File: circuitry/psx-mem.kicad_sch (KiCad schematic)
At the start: 27 parts, among them J1 Conn_01x08, J2 Conn_01x06, U1 PFS154-S16, U2 ZD25WQ16C

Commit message: Generated interactive bill of materials.
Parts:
- TP1, TP10, TP11, TP12, TP2, TP3, TP4, TP5, TP6, TP7, TP8, TP9: now left out of the parts list
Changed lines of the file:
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@@
 		(unit 1)
 		(exclude_from_sim no)
-		(in_bom yes)
+		(in_bom no)
 		(on_board yes)
 		(dnp no)
@@
 		(unit 1)
 		(exclude_from_sim no)
-		(in_bom yes)
+		(in_bom no)
 		(on_board yes)
 		(dnp no)
@@
 		(unit 1)
 		(exclude_from_sim no)
-		(in_bom yes)
+		(in_bom no)
 		(on_board yes)
 		(dnp no)
@@
 		(unit 1)
 		(exclude_from_sim no)
-		(in_bom yes)
+		(in_bom no)
 		(on_board yes)
 		(dnp no)
@@
 		(unit 1)
 		(exclude_from_sim no)
-		(in_bom yes)
+		(in_bom no)
 		(on_board yes)
 		(dnp no)
@@
 		(unit 1)
 		(exclude_from_sim no)
-		(in_bom yes)
+		(in_bom no)
 		(on_board yes)
 		(dnp no)
@@
 		(unit 1)
 		(exclude_from_sim no)
-		(in_bom yes)
+		(in_bom no)
 		(on_board yes)
 		(dnp no)
@@
 		(unit 1)
 		(exclude_from_sim no)
-		(in_bom yes)
+		(in_bom no)
 		(on_board yes)
 		(dnp no)
@@
 		(unit 1)
 		(exclude_from_sim no)
-		(in_bom yes)
+		(in_bom no)
 		(on_board yes)
 		(dnp no)
@@
 		(unit 1)
 		(exclude_from_sim no)
-		(in_bom yes)
+		(in_bom no)
 		(on_board yes)
 		(dnp no)
@@
 		(unit 1)
 		(exclude_from_sim no)
-		(in_bom yes)
+		(in_bom no)
 		(on_board yes)
 		(dnp no)
@@
 		(unit 1)
 		(exclude_from_sim no)
-		(in_bom yes)
-		(on_board yes)
-		(dnp no)
+		(in_bom no)
+		(on_board yes)
+		(dnp no)

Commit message: Updated to use libraries in submodules.
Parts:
- TP1, TP10, TP11, TP12, TP2, TP3, TP4, TP5, TP6, TP7, TP8, TP9: symbol PSX-MEM:TestPoint -> PSX_Memory:TestPoint; now in the parts list
- U1: symbol PSX-MEM:PFS154-S16 -> PSX_Memory:PFS154-S16
- U2: symbol PSX-MEM:ZD25WQ16V -> PSX_Memory:ZD25WQ16V
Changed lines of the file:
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@@
 	)
 	(symbol
-		(lib_id "PSX-MEM:TestPoint")
+		(lib_id "PSX_Memory:TestPoint")
 		(at 154.94 124.46 0)
 		(mirror x)
 		(unit 1)
 		(exclude_from_sim no)
-		(in_bom no)
+		(in_bom yes)
 		(on_board yes)
 		(dnp no)
@@
 	)
 	(symbol
-		(lib_id "PSX-MEM:TestPoint")
+		(lib_id "PSX_Memory:TestPoint")
 		(at 71.12 81.28 0)
 		(unit 1)
 		(exclude_from_sim no)
-		(in_bom no)
+		(in_bom yes)
 		(on_board yes)
 		(dnp no)
@@
 	)
 	(symbol
-		(lib_id "PSX-MEM:TestPoint")
+		(lib_id "PSX_Memory:TestPoint")
 		(at 139.7 124.46 0)
 		(mirror x)
 		(unit 1)
 		(exclude_from_sim no)
-		(in_bom no)
+		(in_bom yes)
 		(on_board yes)
 		(dnp no)
@@
 	)
 	(symbol
-		(lib_id "PSX-MEM:TestPoint")
+		(lib_id "PSX_Memory:TestPoint")
 		(at 78.74 81.28 0)
 		(unit 1)
 		(exclude_from_sim no)
-		(in_bom no)
+		(in_bom yes)
 		(on_board yes)
 		(dnp no)
@@
 	)
 	(symbol
-		(lib_id "PSX-MEM:ZD25WQ16V")
+		(lib_id "PSX_Memory:ZD25WQ16V")
 		(at 121.92 114.3 0)
 		(unit 1)
@@
 	)
 	(symbol
-		(lib_id "PSX-MEM:TestPoint")
+		(lib_id "PSX_Memory:TestPoint")
 		(at 86.36 124.46 180)
 		(unit 1)
 		(exclude_from_sim no)
-		(in_bom no)
+		(in_bom yes)
 		(on_board yes)
 		(dnp no)
@@
 	)
 	(symbol
-		(lib_id "PSX-MEM:TestPoint")
+		(lib_id "PSX_Memory:TestPoint")
 		(at 147.32 124.46 0)
 		(mirror x)
 		(unit 1)
 		(exclude_from_sim no)
-		(in_bom no)
+		(in_bom yes)
 		(on_board yes)
 		(dnp no)
@@
 	)
 	(symbol
-		(lib_id "PSX-MEM:TestPoint")
+		(lib_id "PSX_Memory:TestPoint")
 		(at 63.5 124.46 0)
 		(mirror x)
 		(unit 1)
 		(exclude_from_sim no)
-		(in_bom no)
+		(in_bom yes)
 		(on_board yes)
 		(dnp no)
@@
 	)
 	(symbol
-		(lib_id "PSX-MEM:TestPoint")
+		(lib_id "PSX_Memory:TestPoint")
 		(at 71.12 124.46 0)
 		(mirror x)
 		(unit 1)
 		(exclude_from_sim no)
-		(in_bom no)
+		(in_bom yes)
 		(on_board yes)
 		(dnp no)
@@
 	)
 	(symbol
-		(lib_id "PSX-MEM:TestPoint")
+		(lib_id "PSX_Memory:TestPoint")
 		(at 162.56 124.46 0)
 		(mirror x)
 		(unit 1)
 		(exclude_from_sim no)
-		(in_bom no)
+		(in_bom yes)
 		(on_board yes)
 		(dnp no)
@@
 	)
 	(symbol
-		(lib_id "PSX-MEM:TestPoint")
+		(lib_id "PSX_Memory:TestPoint")
 		(at 93.98 124.46 180)
 		(unit 1)
 		(exclude_from_sim no)
-		(in_bom no)
+		(in_bom yes)
 		(on_board yes)
 		(dnp no)
@@
 	)
 	(symbol
-		(lib_id "PSX-MEM:TestPoint")
+		(lib_id "PSX_Memory:TestPoint")
 		(at 63.5 81.28 0)
 		(unit 1)
 		(exclude_from_sim no)
-		(in_bom no)
+		(in_bom yes)
 		(on_board yes)
 		(dnp no)
@@
 	)
 	(symbol
-		(lib_id "PSX-MEM:TestPoint")
+		(lib_id "PSX_Memory:TestPoint")
 		(at 78.74 124.46 0)
 		(mirror x)
 		(unit 1)
 		(exclude_from_sim no)
-		(in_bom no)
+		(in_bom yes)
 		(on_board yes)
 		(dnp no)
@@
 	)
 	(symbol
-		(lib_id "PSX-MEM:PFS154-S16")
+		(lib_id "PSX_Memory:PFS154-S16")
 		(at 182.88 109.22 0)
 		(mirror y)
@@
 		)
 		(property "Footprint" "Package_SO:SOIC-16_3.9x9.9mm_P1.27mm"
-			(at 191.77 99.06 0)
+			(at 191.77 96.52 0)
 			(effects
 				(font
@@
 		)
 		(property "Datasheet" ""
-			(at 191.77 99.06 0)
-			(effects
-				(font
+			(at 191.77 96.52 0)
+			(effects
+				(font

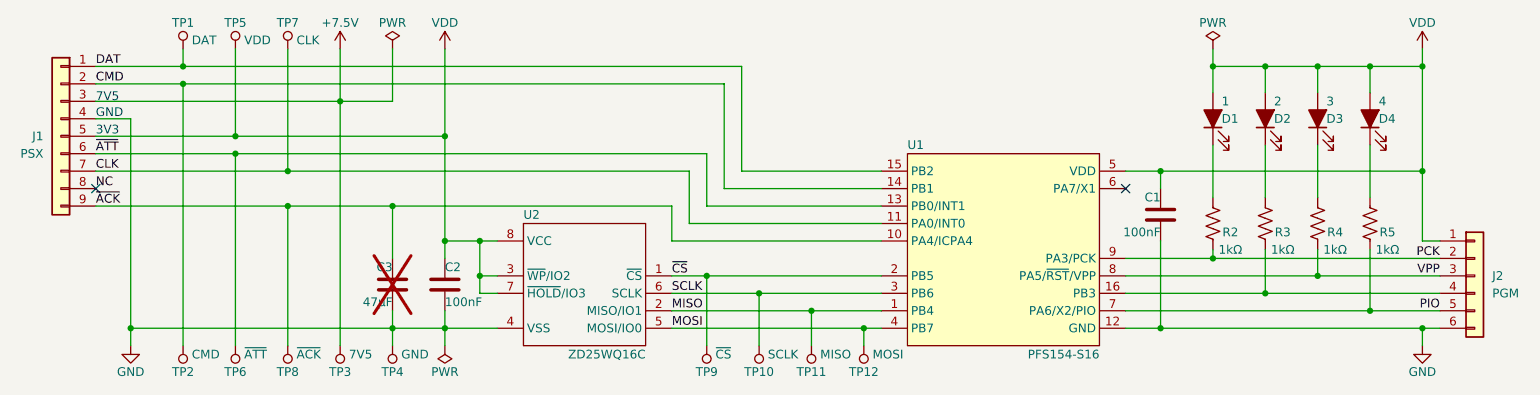
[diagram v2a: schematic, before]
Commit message: Schematic and layout completed.
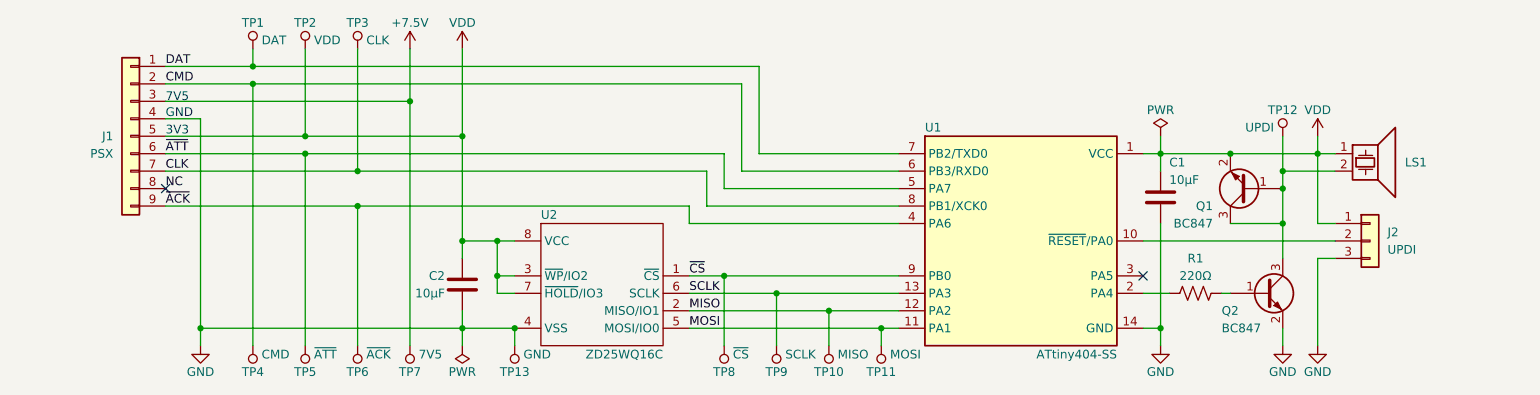
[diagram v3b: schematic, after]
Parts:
- removed C3: 47µF, Capacitor_SMD:C_0805_2012Metric_Pad1.18x1.45mm_HandSolder, symbol Device:C
- removed D1, D2, D3, D4: LED_Filled, LED_SMD:LED_0805_2012Metric_Pad1.15x1.40mm_HandSolder, symbol Device:LED_Filled
- removed J2: Conn_01x06, PSX_MEM:Debug_2x03_P2.54mm, symbol Connector_Generic:Conn_01x06
- removed R2, R3, R4, R5: 1kΩ, Resistor_SMD:R_0805_2012Metric_Pad1.20x1.40mm_HandSolder, symbol Device:R_US
- removed TP4: TestPoint, PSX_MEM:TestPoint, symbol PSX_Memory:TestPoint
- removed U1: PFS154-S16, Package_SO:SOIC-16_3.9x9.9mm_P1.27mm, symbol PSX_Memory:PFS154-S16
- added J2: Conn_01x03, PSX_Memory:TestPoint_UPDI, symbol Connector_Generic:Conn_01x03
- added LS1: Speaker_Crystal, PSX_Memory:BUZ-SMD_4P-L7.5-W7.5-BR, symbol Device:Speaker_Crystal
- added Q1, Q2: BC847, Package_TO_SOT_SMD:SOT-23-3, symbol Transistor_BJT:BC847
- added R1: 220Ω, Resistor_SMD:R_0805_2012Metric, symbol Device:R_US
- added TP12, TP13: TestPoint, TestPoint:TestPoint_Pad_D1.0mm, symbol PSX_Memory:TestPoint
- added U1: ATtiny404-SS, Package_SO:SOIC-14_3.9x8.7mm_P1.27mm, symbol PSX_Memory:ATtiny404-SS
- C1, C2: value 100nF -> 10µF; footprint Capacitor_SMD:C_0805_2012Metric_Pad1.18x1.45mm_HandSolder -> Capacitor_SMD:C_0805_2012Metric
- TP1: footprint PSX_MEM:TestPoint -> TestPoint:TestPoint_Pad_D1.0mm; now left out of the parts list
- TP10: renamed from TP11; footprint PSX_MEM:TestPoint -> TestPoint:TestPoint_Pad_D1.0mm; now left out of the parts list
- TP11: renamed from TP12; footprint PSX_MEM:TestPoint -> TestPoint:TestPoint_Pad_D1.0mm; now left out of the parts list
- TP2: renamed from TP5; footprint PSX_MEM:TestPoint -> TestPoint:TestPoint_Pad_D1.0mm; now left out of the parts list
- TP3: renamed from TP7; footprint PSX_MEM:TestPoint -> TestPoint:TestPoint_Pad_D1.0mm; now left out of the parts list
- TP4: renamed from TP2; footprint PSX_MEM:TestPoint -> TestPoint:TestPoint_Pad_D1.0mm; now left out of the parts list
- TP5: renamed from TP6; footprint PSX_MEM:TestPoint -> TestPoint:TestPoint_Pad_D1.0mm; now left out of the parts list
- TP6: renamed from TP8; footprint PSX_MEM:TestPoint -> TestPoint:TestPoint_Pad_D1.0mm; now left out of the parts list
- TP7: renamed from TP3; footprint PSX_MEM:TestPoint -> TestPoint:TestPoint_Pad_D1.0mm; now left out of the parts list
- TP8: renamed from TP9; footprint PSX_MEM:TestPoint -> TestPoint:TestPoint_Pad_D1.0mm; now left out of the parts list
- TP9: renamed from TP10; footprint PSX_MEM:TestPoint -> TestPoint:TestPoint_Pad_D1.0mm; now left out of the parts list
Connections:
- net CLK: now also U1.8 (PB1/XCK0)
- net CMD: now also U1.6 (PB3/RXD0)
- net DAT: now also U1.7 (PB2/TXD0)
- net GND: now also J2.3 (Pin_3), Q2.2 (E), TP13.1, U1.14 (GND)
- net MISO: now also U1.12 (PA2)
- net MOSI: now also U1.11 (PA1)
- net SCLK: now also U1.13 (PA3)
- net VDD: now also J2.1 (Pin_1), LS1.1, Q1.2 (E), U1.1 (VCC)
- net ~{ACK}: now also U1.4 (PA6)
- net ~{ATT}: now also U1.5 (PA7)
- net ~{CS}: now also U1.9 (PB0)
- new net: J2.2 (Pin_2), U1.10 (~{RESET}/PA0)
- new net: Q2.1 (B), R1.2
- new net: LS1.2, Q1.1 (B), Q1.3 (C), Q2.3 (C), TP12.1
- new net: R1.1, U1.2 (PA4)
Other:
- moved on the sheet: C1, C2, J1, TP1, TP10, TP11, TP2, TP3, TP4, TP5, TP6, TP7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
